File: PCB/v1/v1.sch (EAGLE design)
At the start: 43 parts, among them U2 AT24C512C-SHD-B

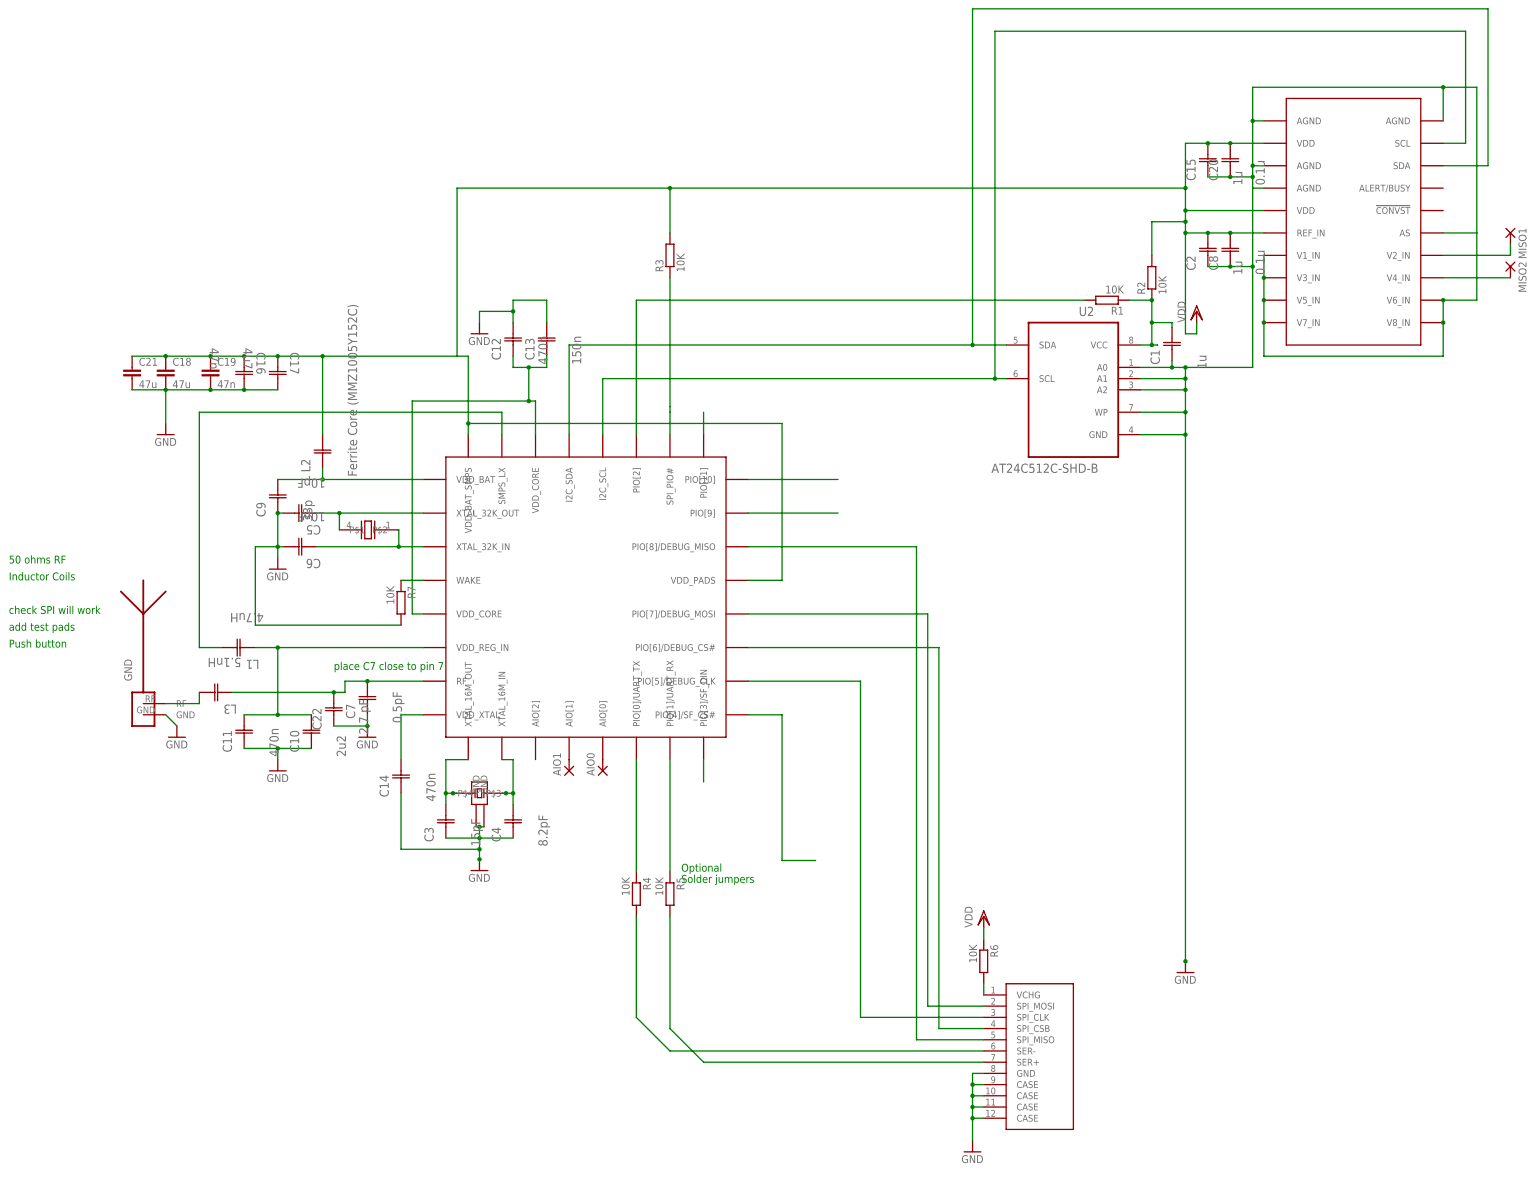
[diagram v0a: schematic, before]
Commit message: final check and submit
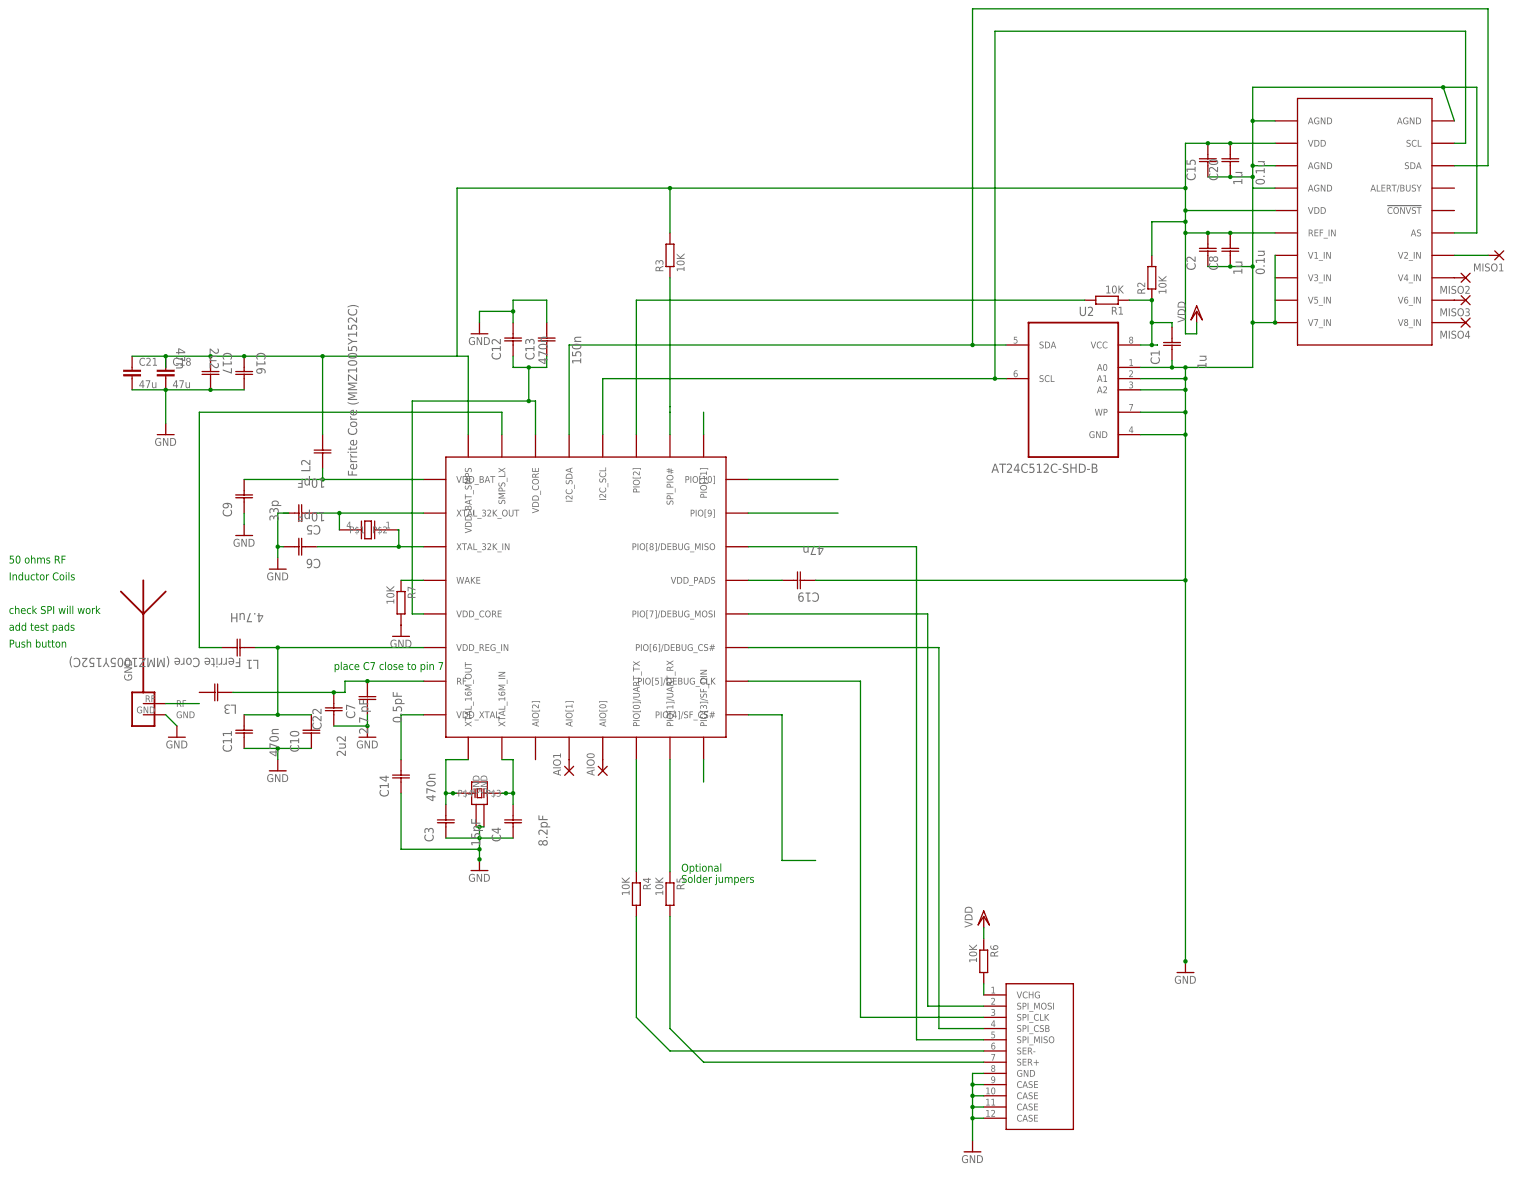
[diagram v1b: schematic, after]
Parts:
- added MISO3, MISO4: (no value), wirepad:1,6/0,8
- C16: value 47n -> 2u2
- C17: value 4u7 -> 47n
- C19: device rcl:C-EUC0402 -> AVX_By_element14_Batch_1:UQCL2A100JAT2A/500
- L3: value 5.1nH -> Ferrite Core (MMZ1005Y152C); device AVX_By_element14_Batch_1:12107C102JAT2A -> AVX_By_element14_Batch_1:UQCL2A100JAT2A/500
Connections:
- removed net N$34: L3.C2
- new net N$73: MISO3.P, U$5.V6_IN
- new net N$83: MISO4.P, U$5.V8_IN
- new net N$87: C19.C2, U$1.VDD_PADS
- net GND: now also C19.C1; no longer C19.2, C5.C2, U$5.V3_IN, U$5.V5_IN, U$5.V6_IN, U$5.V8_IN
- net VDD: no longer C19.1, U$1.VDD_PADS
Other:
- moved on the sheet: C17, C9, MISO1, MISO2
